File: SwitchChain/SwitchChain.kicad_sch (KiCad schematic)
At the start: 1 part, among them J101 Conn_01x06

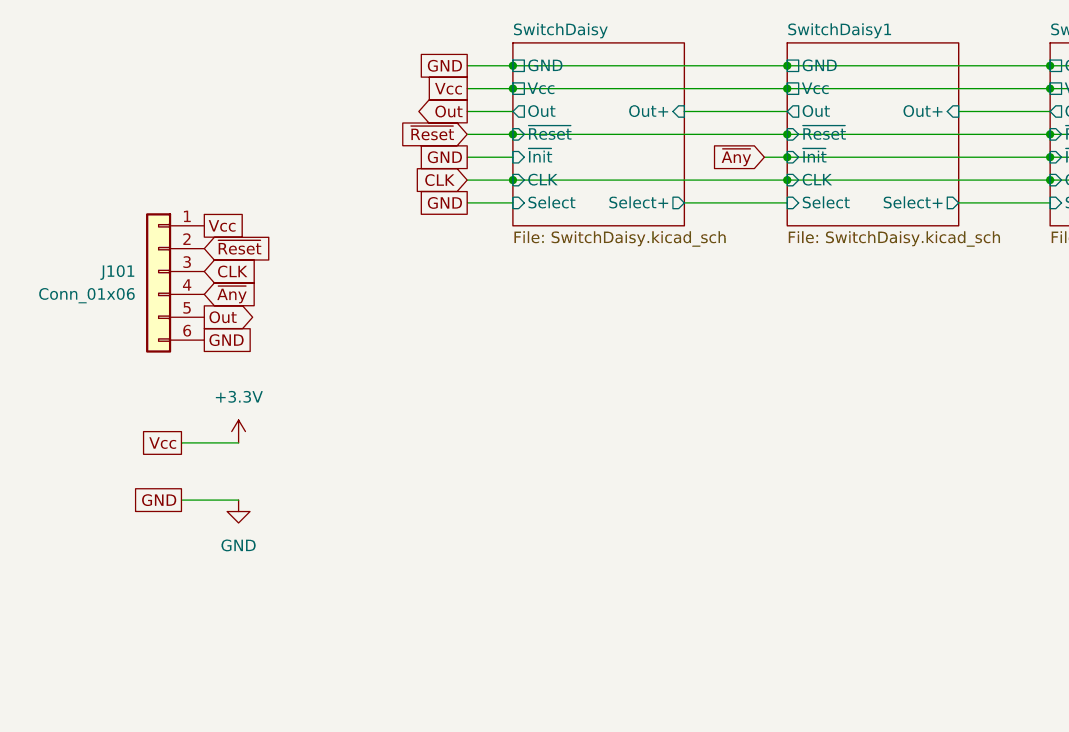
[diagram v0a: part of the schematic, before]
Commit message: fix circuit
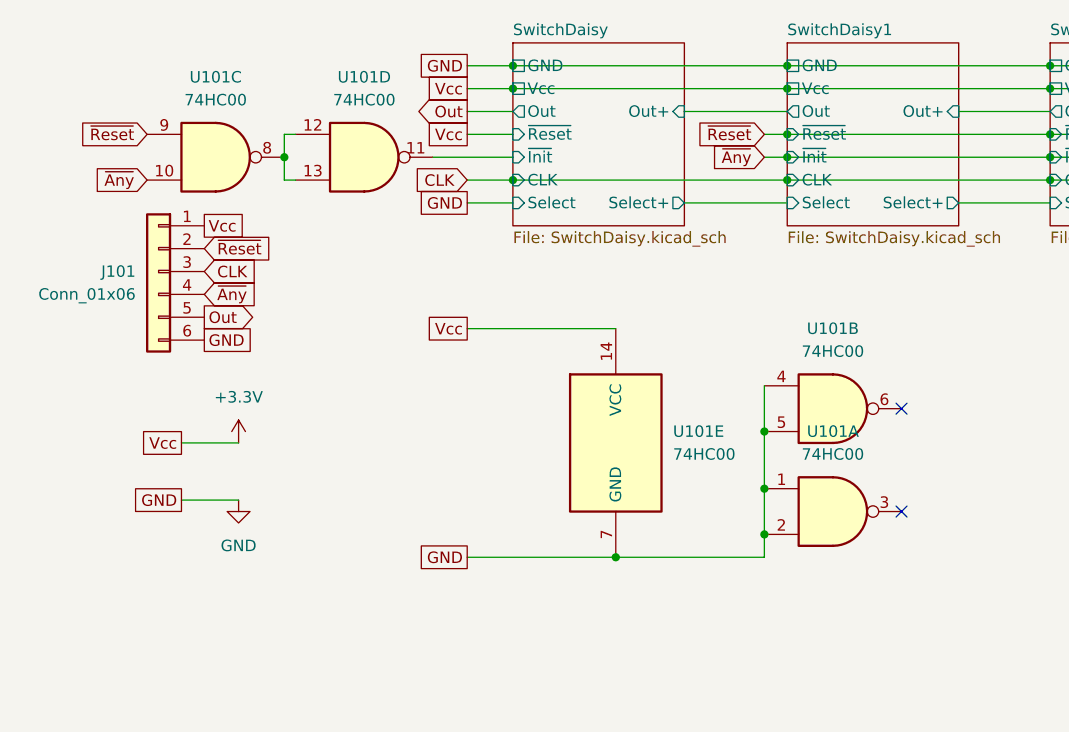
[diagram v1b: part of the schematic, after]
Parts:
- added U101: 74HC00, Package_DFN_QFN:WQFN-14-1EP_2.5x2.5mm_P0.5mm_EP1.45x1.45mm, symbol 74xx:74HC00
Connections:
- net +3.3V: now also U101.14 (VCC)
- net GND: now also U101.1, U101.2, U101.4, U101.5, U101.7 (GND)
- net ~{Any}: now also U101.10
- net ~{Reset}: now also U101.9
- new net: U101.12, U101.13, U101.8
- new net SwitchDaisy/~{Init}: U101.11
- no-connect marks 2 -> 4
